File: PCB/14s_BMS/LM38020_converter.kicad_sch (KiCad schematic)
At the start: 4 parts, among them U3 LMR38020FDDAR

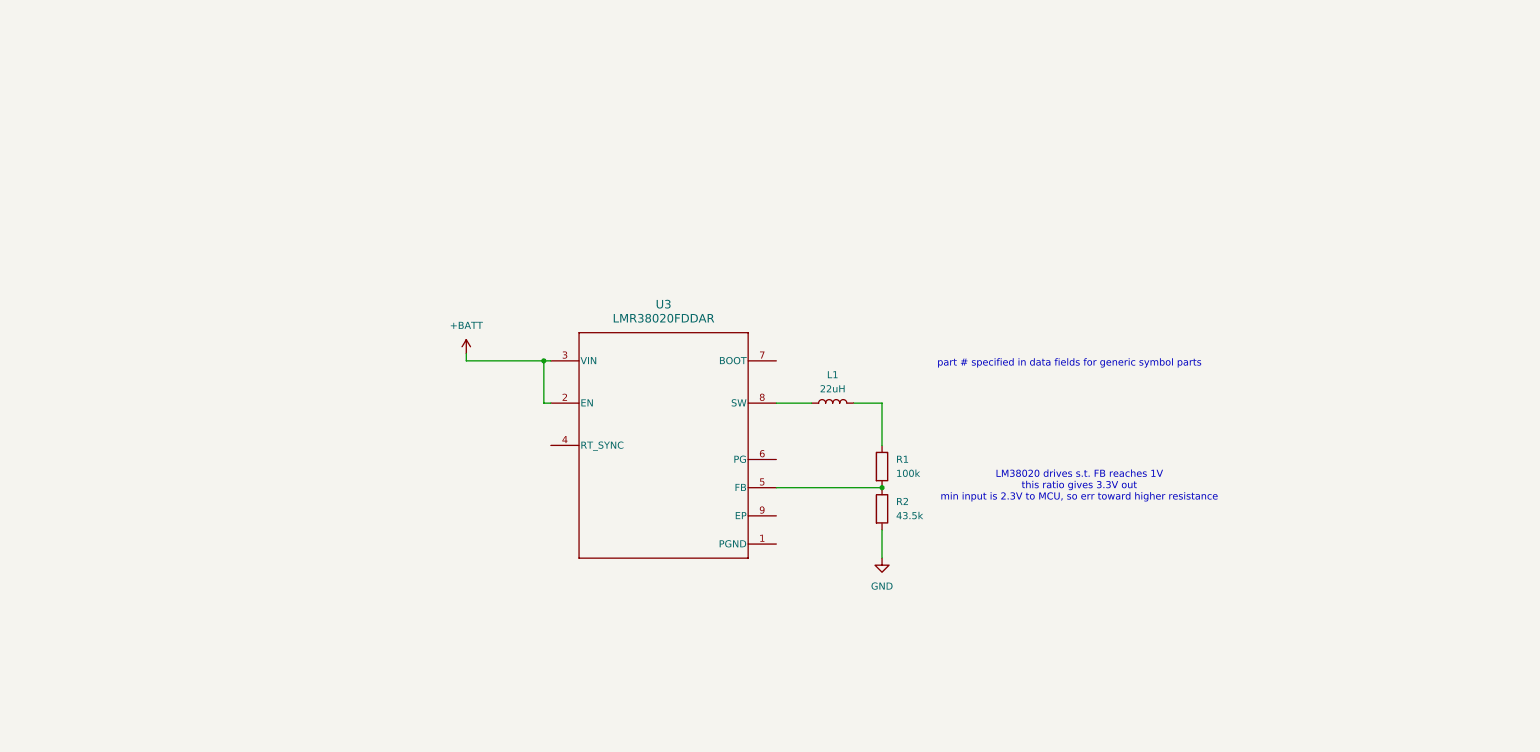
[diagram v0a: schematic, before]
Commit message: rev 1 of power supply design
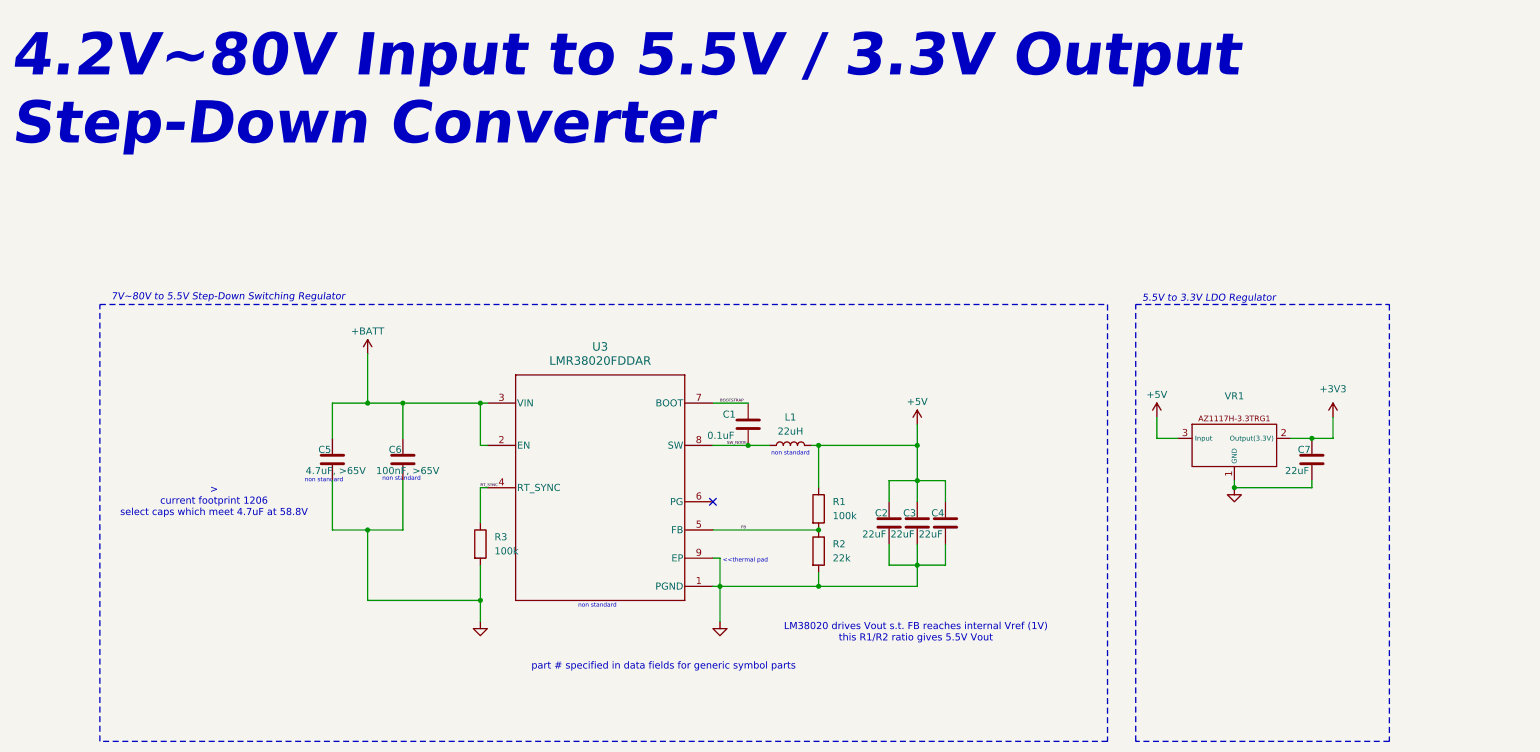
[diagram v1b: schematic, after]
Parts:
- added C1: 0.1uF, Capacitor_SMD:C_0402_1005Metric_Pad0.74x0.62mm_HandSolder, symbol Device:C
- added C2, C3, C4, C7: 22uF, Capacitor_SMD:C_0805_2012Metric_Pad1.18x1.45mm_HandSolder, symbol Device:C
- added C5: 4.7uF, >65V, Capacitor_SMD:C_1206_3216Metric_Pad1.33x1.80mm_HandSolder, symbol Device:C
- added C6: 100nF, >65V, Capacitor_SMD:C_1206_3216Metric_Pad1.33x1.80mm_HandSolder, symbol Device:C
- added R3: 100k, Resistor_SMD:R_0402_1005Metric_Pad0.72x0.64mm_HandSolder, symbol Device:R
- added VR1: ~, Package_TO_SOT_SMD:SOT-223-3_TabPin2, symbol 0_PMIC:AZ1117H-3.3TRG1
- R1: footprint Resistor_SMD:R_0603_1608Metric -> Resistor_SMD:R_0402_1005Metric_Pad0.72x0.64mm_HandSolder; Part 0603WAF1003T5E -> 0402WGF1003TCE
- R2: value 43.5k -> 22k; Part 0603WAF1003T5E -> 0402WGF2202TCE
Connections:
- net +BATT: now also C5.1, C6.1
- net GND: now also U3.1 (PGND), U3.9 (EP), C2.2, C3.2, C4.2, C5.2, C6.2, C7.2, R3.2, VR1.1 (GND)
- net +5V: now reaches L1.2, R1.1
- net +5V: now also C2.1, C3.1, C4.1, VR1.3 (Input)
- net FB: now reaches R1.2, R2.1, U3.5 (FB)
- net RT_SYNC: now reaches U3.4 (RT_SYNC)
- net RT_SYNC: now also R3.1
- net BOOTSTRAP: now reaches U3.7 (BOOT)
- net BOOTSTRAP: now also C1.1
- net SW_NODE: now reaches L1.1, U3.8 (SW)
- net SW_NODE: now also C1.2
- new net +3V3: C7.1, VR1.2 (Output(3.3V))
- no-connect marks 0 -> 1
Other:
- note added: "4.2V~80V Input to 5.5V / 3.3V Output Step-Down Converter"
- note added: "5.5V to 3.3V LDO Regulator"
- note added: "7V~80V to 5.5V Step-Down Switching Regulator"
- note added: "<<thermal pad"
- note added: "> current footprint 1206 select caps which meet 4.7uF at 58.8V"
- note added: "LM38020 drives Vout s.t. FB reaches internal Vref (1V) this R1/R2 ratio gives 5.5V Vout"
- note added: "non standard"
- note removed: "LM38020 drives s.t. FB reaches 1V this ratio gives 3.3V out min input is 2.3V to MCU, so err toward higher resistance"
- company: (none) -> Hayden Higgins
- title: (none) -> LM38020 Converter
- moved on the sheet: L1, R1, R2, U3
